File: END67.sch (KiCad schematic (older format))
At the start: 14 parts

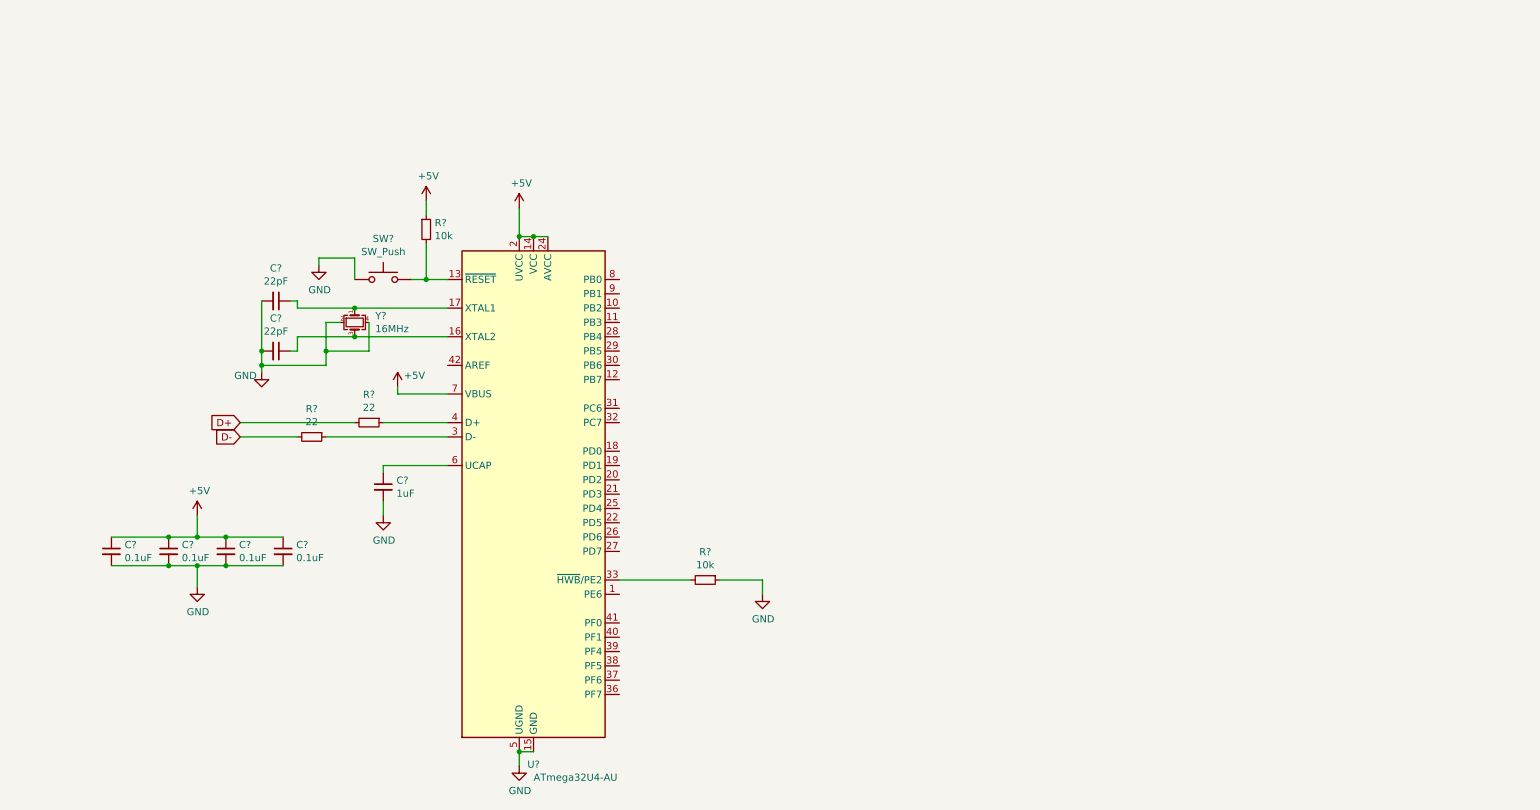
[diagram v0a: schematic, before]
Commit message: Finished Layout
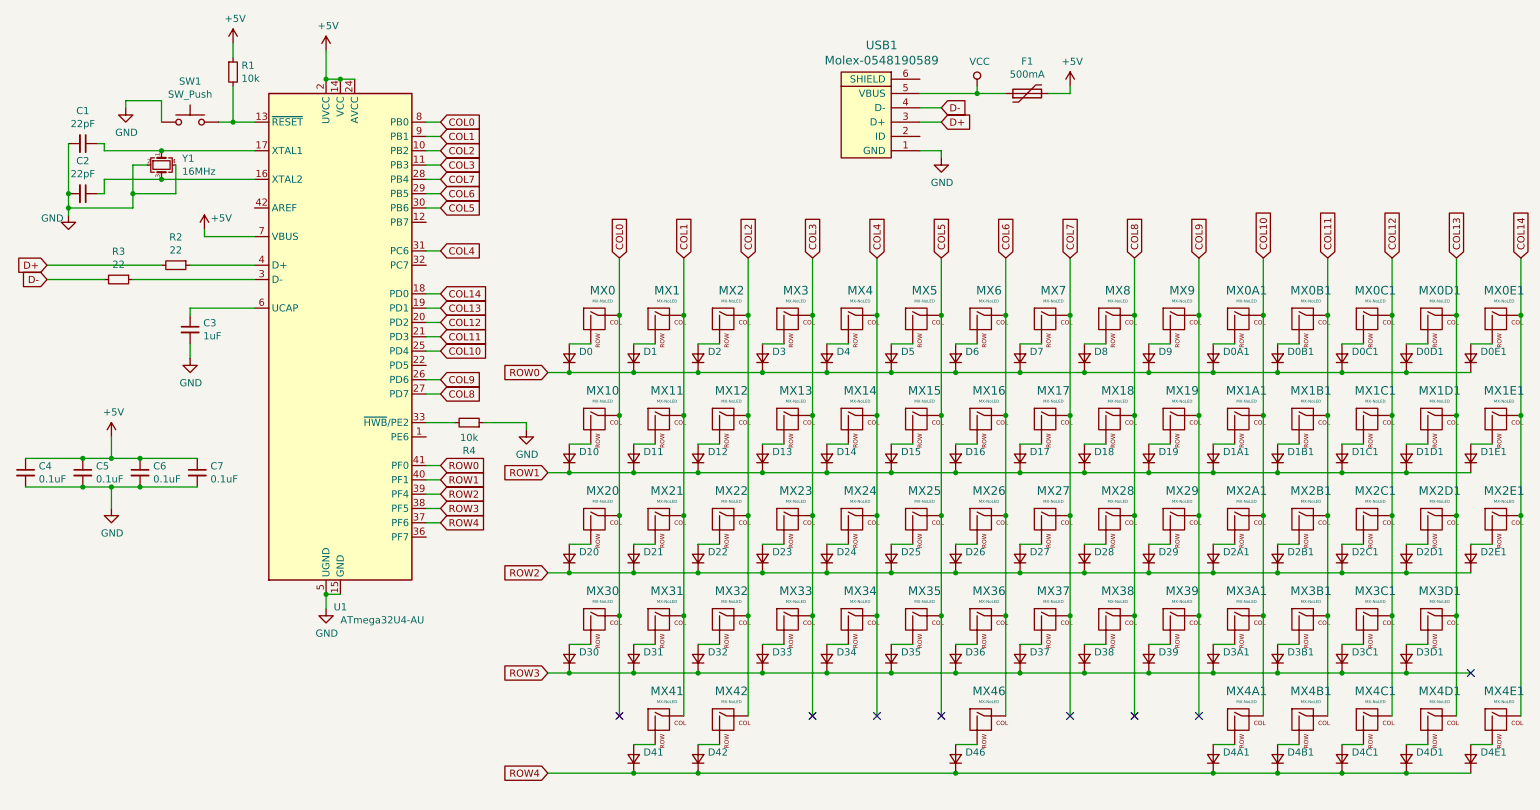
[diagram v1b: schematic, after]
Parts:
- added D0, D0A1, D0B1, D0C1, D0D1, D0E1, D1, D10, D11, D12, D13, D14, D15, D16, D17, D18, D19, D1A1, D1B1, D1C1, D1D1, D1E1, D2, D20, D21, D22, D23, D24, D25, D26, D27, D28, D29, D2A1, D2B1, D2C1, D2D1, D2E1, D3, D30, D31, D32, D33, D34, D35, D36, D37, D38, D39, D3A1, D3B1, D3C1, D3D1, D4, D41, D42, D46, D4A1, D4B1, D4C1, D4D1, D4E1, D5, D6, D7, D8, D9: D_Small, Diode_SMD:D_SOD-123, symbol Device:D_Small
- added F1: 500mA, Fuse:Fuse_1206_3216Metric_Pad1.42x1.75mm_HandSolder, symbol Device:Polyfuse
- added MX0, MX0A1, MX0B1, MX0C1, MX0D1, MX1, MX10, MX12, MX13, MX14, MX15, MX16, MX17, MX18, MX19, MX1A1, MX1B1, MX1C1, MX1D1, MX2, MX20, MX22, MX23, MX24, MX25, MX26, MX27, MX28, MX29, MX2A1, MX2B1, MX2C1, MX2E1, MX3, MX30, MX32, MX33, MX34, MX35, MX36, MX37, MX38, MX39, MX3A1, MX3B1, MX3D1, MX4, MX4C1, MX4D1, MX4E1, MX5, MX6, MX7, MX8, MX9: MX-NoLED, MX_Alps_Hybrid_SW:MX-1U-NoLED, symbol MX_Alps_Hybrid:MX-NoLED
- added MX0E1: MX-NoLED, MX_Alps_Hybrid_SW:MX-2U-NoLED, symbol MX_Alps_Hybrid:MX-NoLED
- added MX11, MX1E1: MX-NoLED, MX_Alps_Hybrid_SW:MX-1.5U-NoLED, symbol MX_Alps_Hybrid:MX-NoLED
- added MX21, MX3C1: MX-NoLED, MX_Alps_Hybrid_SW:MX-1.75U-NoLED, symbol MX_Alps_Hybrid:MX-NoLED
- added MX2D1, MX31: MX-NoLED, MX_Alps_Hybrid_SW:MX-2.25U-NoLED, symbol MX_Alps_Hybrid:MX-NoLED
- added MX41, MX42, MX4A1, MX4B1: MX-NoLED, MX_Alps_Hybrid_SW:MX-1.25U-NoLED, symbol MX_Alps_Hybrid:MX-NoLED
- added MX46: MX-NoLED, MX_Alps_Hybrid_SW:MX-6.25U-NoLED, symbol MX_Alps_Hybrid:MX-NoLED
- added USB1: Molex-0548190589, random-keyboard-parts:Molex-0548190589, symbol random-keyboard-parts:Molex-0548190589
- C1, C2, C3, C4, C5, C6, C7: renamed from C?; footprint (none) -> Capacitor_SMD:C_0805_2012Metric_Pad1.15x1.40mm_HandSolder
- R1, R2, R3, R4: renamed from R?; footprint (none) -> Resistor_SMD:R_0805_2012Metric_Pad1.15x1.40mm_HandSolder
- SW1: renamed from SW?; footprint (none) -> random-keyboard-parts:SKQG-1155865
- Y1: renamed from Y?; footprint (none) -> Crystal:Crystal_SMD_3225-4Pin_3.2x2.5mm_HandSoldering
- gave numbers to parts that had none: 1
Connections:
- net +5V: now also F1.2
- net D+: now also USB1.3 (D+)
- net D-: now also USB1.4 (D-)
- net GND: now also USB1.1 (GND)
- net COL2: now reaches U1.10 (PB2)
- net COL2: now also MX12.1 (COL), MX2.1 (COL), MX22.1 (COL), MX32.1 (COL), MX42.1 (COL)
- net COL3: now reaches U1.11 (PB3)
- net COL3: now also MX13.1 (COL), MX23.1 (COL), MX3.1 (COL), MX33.1 (COL)
- net COL14: now reaches U1.18 (PD0)
- net COL14: now also MX0E1.1 (COL), MX1E1.1 (COL), MX2E1.1 (COL), MX4E1.1 (COL)
- net COL13: now reaches U1.19 (PD1)
- net COL13: now also MX0D1.1 (COL), MX1D1.1 (COL), MX2D1.1 (COL), MX3D1.1 (COL), MX4D1.1 (COL)
- net COL12: now reaches U1.20 (PD2)
- net COL12: now also MX0C1.1 (COL), MX1C1.1 (COL), MX2C1.1 (COL), MX3C1.1 (COL), MX4C1.1 (COL)
- net COL11: now reaches U1.21 (PD3)
- net COL11: now also MX0B1.1 (COL), MX1B1.1 (COL), MX2B1.1 (COL), MX3B1.1 (COL), MX4B1.1 (COL)
- net COL10: now reaches U1.25 (PD4)
- net COL10: now also MX0A1.1 (COL), MX1A1.1 (COL), MX2A1.1 (COL), MX3A1.1 (COL), MX4A1.1 (COL)
- net COL9: now reaches U1.26 (PD6)
- net COL9: now also MX19.1 (COL), MX29.1 (COL), MX39.1 (COL), MX9.1 (COL)
- net COL8: now reaches U1.27 (PD7)
- net COL8: now also MX18.1 (COL), MX28.1 (COL), MX38.1 (COL), MX8.1 (COL)
- net COL7: now reaches U1.28 (PB4)
- net COL7: now also MX17.1 (COL), MX27.1 (COL), MX37.1 (COL), MX7.1 (COL)
- net COL6: now reaches U1.29 (PB5)
- net COL6: now also MX16.1 (COL), MX26.1 (COL), MX36.1 (COL), MX46.1 (COL), MX6.1 (COL)
- net COL5: now reaches U1.30 (PB6)
- net COL5: now also MX15.1 (COL), MX25.1 (COL), MX35.1 (COL), MX5.1 (COL)
- net COL4: now reaches U1.31 (PC6)
- net COL4: now also MX14.1 (COL), MX24.1 (COL), MX34.1 (COL), MX4.1 (COL)
- net ROW4: now reaches U1.37 (PF6)
- net ROW4: now also D41.1 (K), D42.1 (K), D46.1 (K), D4A1.1 (K), D4B1.1 (K), D4C1.1 (K), D4D1.1 (K), D4E1.1 (K)
- net ROW3: now reaches U1.38 (PF5)
- net ROW3: now also D30.1 (K), D31.1 (K), D32.1 (K), D33.1 (K), D34.1 (K), D35.1 (K), D36.1 (K), D37.1 (K), D38.1 (K), D39.1 (K), D3A1.1 (K), D3B1.1 (K), D3C1.1 (K), D3D1.1 (K)
- net ROW2: now reaches U1.39 (PF4)
- net ROW2: now also D20.1 (K), D21.1 (K), D22.1 (K), D23.1 (K), D24.1 (K), D25.1 (K), D26.1 (K), D27.1 (K), D28.1 (K), D29.1 (K), D2A1.1 (K), D2B1.1 (K), D2C1.1 (K), D2D1.1 (K), D2E1.1 (K)
- net ROW1: now reaches U1.40 (PF1)
- net ROW1: now also D10.1 (K), D11.1 (K), D12.1 (K), D13.1 (K), D14.1 (K), D15.1 (K), D16.1 (K), D17.1 (K), D18.1 (K), D19.1 (K), D1A1.1 (K), D1B1.1 (K), D1C1.1 (K), D1D1.1 (K), D1E1.1 (K)
- net ROW0: now reaches U1.41 (PF0)
- net ROW0: now also D0.1 (K), D0A1.1 (K), D0B1.1 (K), D0C1.1 (K), D0D1.1 (K), D0E1.1 (K), D1.1 (K), D2.1 (K), D3.1 (K), D4.1 (K), D5.1 (K), D6.1 (K), D7.1 (K), D8.1 (K), D9.1 (K)
- net COL0: now reaches U1.8 (PB0)
- net COL0: now also MX0.1 (COL), MX10.1 (COL), MX20.1 (COL), MX30.1 (COL)
- net COL1: now reaches U1.9 (PB1)
- net COL1: now also MX1.1 (COL), MX11.1 (COL), MX21.1 (COL), MX31.1 (COL), MX41.1 (COL)
- new net: D4.2 (A), MX4.2 (ROW)
- new net: D5.2 (A), MX5.2 (ROW)
- new net: D6.2 (A), MX6.2 (ROW)
- new net: D7.2 (A), MX7.2 (ROW)
- new net: D8.2 (A), MX8.2 (ROW)
- new net: D9.2 (A), MX9.2 (ROW)
- new net: D0A1.2 (A), MX0A1.2 (ROW)
- new net: D0B1.2 (A), MX0B1.2 (ROW)
- new net: D0C1.2 (A), MX0C1.2 (ROW)
- new net: D0D1.2 (A), MX0D1.2 (ROW)
- new net: D0E1.2 (A), MX0E1.2 (ROW)
- new net: D3.2 (A), MX3.2 (ROW)
- new net: D2.2 (A), MX2.2 (ROW)
- new net: D1.2 (A), MX1.2 (ROW)
- new net: D0.2 (A), MX0.2 (ROW)
- new net: D14.2 (A), MX14.2 (ROW)
- new net: D15.2 (A), MX15.2 (ROW)
- new net: D16.2 (A), MX16.2 (ROW)
- new net: D17.2 (A), MX17.2 (ROW)
- new net: D18.2 (A), MX18.2 (ROW)
- new net: D19.2 (A), MX19.2 (ROW)
- new net: D1A1.2 (A), MX1A1.2 (ROW)
- new net: D1B1.2 (A), MX1B1.2 (ROW)
- new net: D1C1.2 (A), MX1C1.2 (ROW)
- new net: D1D1.2 (A), MX1D1.2 (ROW)
- new net: D1E1.2 (A), MX1E1.2 (ROW)
- new net: D13.2 (A), MX13.2 (ROW)
- new net: D12.2 (A), MX12.2 (ROW)
- new net: D11.2 (A), MX11.2 (ROW)
- new net: D10.2 (A), MX10.2 (ROW)
- new net: D24.2 (A), MX24.2 (ROW)
- new net: D25.2 (A), MX25.2 (ROW)
- new net: D26.2 (A), MX26.2 (ROW)
- new net: D27.2 (A), MX27.2 (ROW)
- new net: D28.2 (A), MX28.2 (ROW)
- new net: D29.2 (A), MX29.2 (ROW)
- new net: D2A1.2 (A), MX2A1.2 (ROW)
- new net: D2B1.2 (A), MX2B1.2 (ROW)
- new net: D2C1.2 (A), MX2C1.2 (ROW)
- new net: D2D1.2 (A), MX2D1.2 (ROW)
- new net: D2E1.2 (A), MX2E1.2 (ROW)
- new net: D23.2 (A), MX23.2 (ROW)
- new net: D22.2 (A), MX22.2 (ROW)
- new net: D21.2 (A), MX21.2 (ROW)
- new net: D20.2 (A), MX20.2 (ROW)
- new net: D34.2 (A), MX34.2 (ROW)
- new net: D35.2 (A), MX35.2 (ROW)
- new net: D36.2 (A), MX36.2 (ROW)
- new net: D37.2 (A), MX37.2 (ROW)
- new net: D38.2 (A), MX38.2 (ROW)
- new net: D39.2 (A), MX39.2 (ROW)
- new net: D3A1.2 (A), MX3A1.2 (ROW)
- new net: D3B1.2 (A), MX3B1.2 (ROW)
- new net: D3C1.2 (A), MX3C1.2 (ROW)
- new net: D3D1.2 (A), MX3D1.2 (ROW)
- new net: D33.2 (A), MX33.2 (ROW)
- new net: D32.2 (A), MX32.2 (ROW)
- new net: D31.2 (A), MX31.2 (ROW)
- new net: D30.2 (A), MX30.2 (ROW)
- new net: D46.2 (A), MX46.2 (ROW)
- new net: D4A1.2 (A), MX4A1.2 (ROW)
- new net: D4B1.2 (A), MX4B1.2 (ROW)
- new net: D4C1.2 (A), MX4C1.2 (ROW)
- new net: D4D1.2 (A), MX4D1.2 (ROW)
- new net: D4E1.2 (A), MX4E1.2 (ROW)
- new net: D42.2 (A), MX42.2 (ROW)
- new net: D41.2 (A), MX41.2 (ROW)
- new net VCC: F1.1, USB1.5 (VBUS)
- no-connect marks 0 -> 8
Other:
- moved on the sheet: C1, C2, C3, C4, C5, C6, C7, R1, R2, R3, R4, SW1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

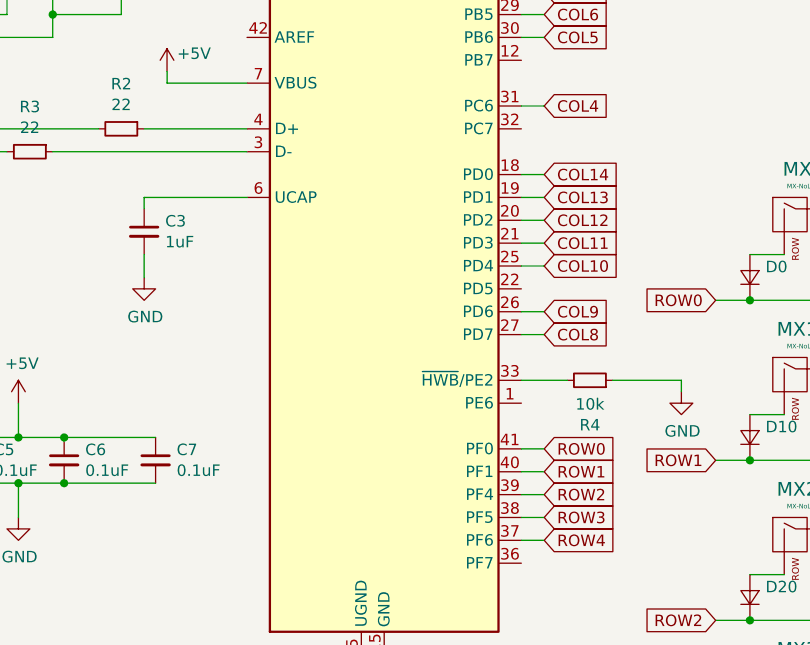
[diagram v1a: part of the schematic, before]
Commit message: Finished First Prototype
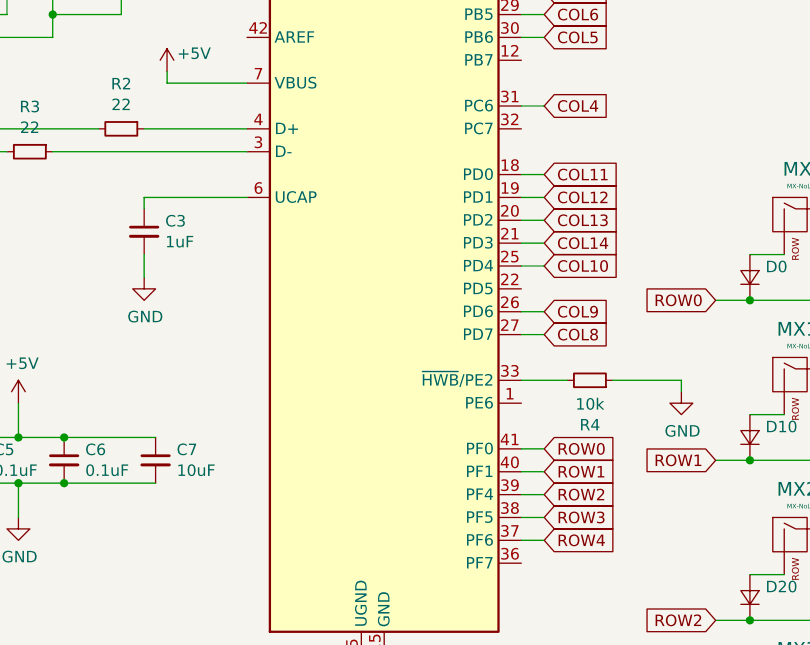
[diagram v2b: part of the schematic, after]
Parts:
- C7: value 0.1uF -> 10uF
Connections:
- net COL11: now also U1.18 (PD0); no longer U1.21 (PD3)
- net COL12: now also U1.19 (PD1); no longer U1.20 (PD2)
- net COL13: now also U1.20 (PD2); no longer U1.19 (PD1)
- net COL14: now also U1.21 (PD3); no longer U1.18 (PD0)
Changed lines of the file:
@@
 P 1750 3750
 F 0 "C7" H 1842 3796 50  0000 L CNN
-F 1 "0.1uF" H 1842 3705 50  0000 L CNN
+F 1 "10uF" H 1842 3705 50  0000 L CNN
 F 2 "Capacitor_SMD:C_0805_2012Metric_Pad1.15x1.40mm_HandSolder" H 1750 3750 50  0001 C CNN
 F 3 "~" H 1750 3750 50  0001 C CNN
@@
 Wire Wire Line
 	3350 3700 3450 3700
+Text GLabel 3450 2800 2    50   Input ~ 0
+COL14
+Text GLabel 3450 2700 2    50   Input ~ 0
+COL13
+Text GLabel 3450 2600 2    50   Input ~ 0
+COL12
 Text GLabel 3450 2500 2    50   Input ~ 0
-COL14
-Text GLabel 3450 2600 2    50   Input ~ 0
-COL13
-Text GLabel 3450 2700 2    50   Input ~ 0
-COL12
-Text GLabel 3450 2800 2    50   Input ~ 0
 COL11
 Text GLabel 3450 2900 2    50   Input ~ 0
